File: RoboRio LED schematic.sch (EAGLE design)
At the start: 5 parts

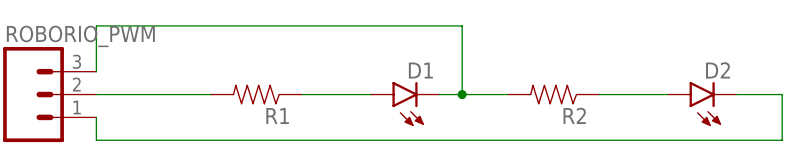
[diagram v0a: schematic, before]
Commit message: Jordan - RoboRio LED fixed
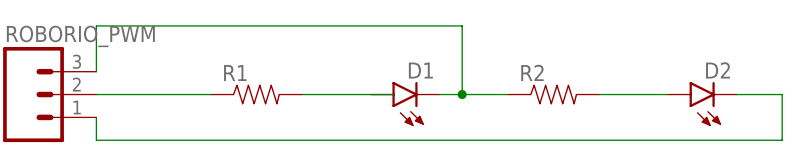
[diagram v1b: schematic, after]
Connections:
- removed net 6V: R1.2, ROBORIO_PWM.2
- removed net N$3: D2.A, R2.1
- new net N$2: R1.2
- new net N$4: D2.A, R2.2
- net N$1: now also ROBORIO_PWM.2; no longer D1.A
- net S: now also R2.1; no longer R2.2
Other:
- moved on the sheet: R1, R2
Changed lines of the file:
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@@
 <instance part="D1" gate="G$1" x="-12.7" y="60.96" rot="R90"/>
 <instance part="D2" gate="G$1" x="20.32" y="60.96" rot="R90"/>
-<instance part="R1" gate="G$1" x="-27.94" y="60.96" rot="R180"/>
-<instance part="R2" gate="G$1" x="5.08" y="60.96" rot="R180"/>
+<instance part="R1" gate="G$1" x="-27.94" y="60.96"/>
+<instance part="R2" gate="G$1" x="5.08" y="60.96"/>
 </instances>
 <busses>
 </busses>
 <nets>
-<net name="N$1" class="0">
-<segment>
-<pinref part="R1" gate="G$1" pin="1"/>
-<pinref part="D1" gate="G$1" pin="A"/>
-<wire x1="-22.86" y1="60.96" x2="-15.24" y2="60.96" width="0.1524" layer="91"/>
-</segment>
-</net>
 <net name="S" class="0">
 <segment>
-<pinref part="D1" gate="G$1" pin="C"/>
-<pinref part="R2" gate="G$1" pin="2"/>
-<wire x1="-7.62" y1="60.96" x2="-5.08" y2="60.96" width="0.1524" layer="91"/>
 <pinref part="ROBORIO_PWM" gate="J$1" pin="3"/>
-<wire x1="-5.08" y1="60.96" x2="0" y2="60.96" width="0.1524" layer="91"/>
 <wire x1="-45.72" y1="63.5" x2="-45.72" y2="68.58" width="0.1524" layer="91"/>
 <wire x1="-45.72" y1="68.58" x2="-5.08" y2="68.58" width="0.1524" layer="91"/>
+<pinref part="D1" gate="G$1" pin="C"/>
+<pinref part="R2" gate="G$1" pin="1"/>
+<wire x1="-7.62" y1="60.96" x2="-5.08" y2="60.96" width="0.1524" layer="91"/>
+<wire x1="-5.08" y1="60.96" x2="0" y2="60.96" width="0.1524" layer="91"/>
 <wire x1="-5.08" y1="68.58" x2="-5.08" y2="60.96" width="0.1524" layer="91"/>
 <junction x="-5.08" y="60.96"/>
-</segment>
-</net>
-<net name="N$3" class="0">
-<segment>
-<pinref part="R2" gate="G$1" pin="1"/>
-<pinref part="D2" gate="G$1" pin="A"/>
-<wire x1="10.16" y1="60.96" x2="17.78" y2="60.96" width="0.1524" layer="91"/>
-</segment>
-</net>
-<net name="6V" class="0">
-<segment>
-<pinref part="ROBORIO_PWM" gate="J$1" pin="2"/>
-<pinref part="R1" gate="G$1" pin="2"/>
-<wire x1="-45.72" y1="60.96" x2="-33.02" y2="60.96" width="0.1524" layer="91"/>
 </segment>
 </net>
@@
 </segment>
 </net>
+<net name="N$1" class="0">
+<segment>
+<pinref part="ROBORIO_PWM" gate="J$1" pin="2"/>
+<pinref part="R1" gate="G$1" pin="1"/>
+<wire x1="-45.72" y1="60.96" x2="-33.02" y2="60.96" width="0.1524" layer="91"/>
+</segment>
+</net>
+<net name="N$2" class="0">
+<segment>
+<pinref part="R1" gate="G$1" pin="2"/>
+<wire x1="-22.86" y1="60.96" x2="-12.7" y2="60.96" width="0.1524" layer="91"/>
+</segment>
+</net>
+<net name="N$4" class="0">
+<segment>
+<pinref part="R2" gate="G$1" pin="2"/>
+<pinref part="D2" gate="G$1" pin="A"/>
+<wire x1="10.16" y1="60.96" x2="17.78" y2="60.96" width="0.1524" layer="91"/>
+</segment>
+</net>

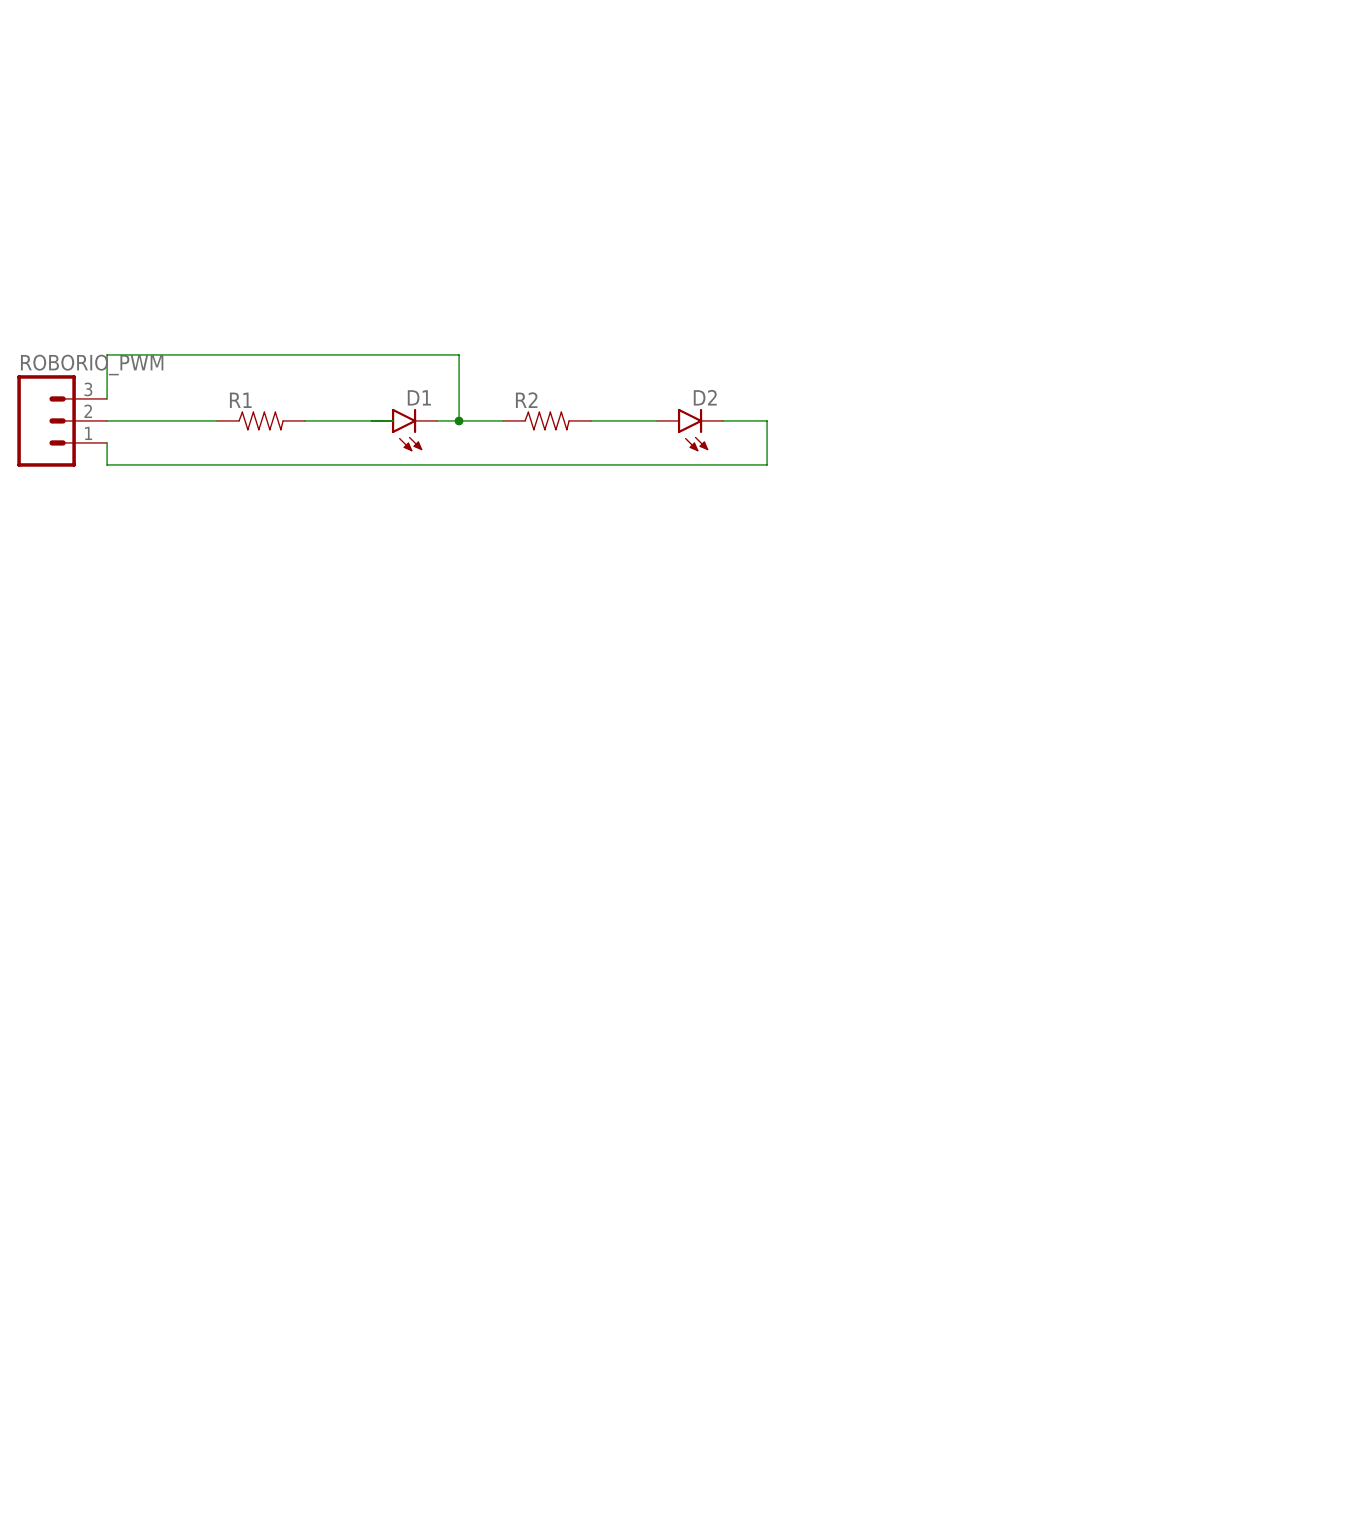
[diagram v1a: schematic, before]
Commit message: Jordan RoboRio LED Final
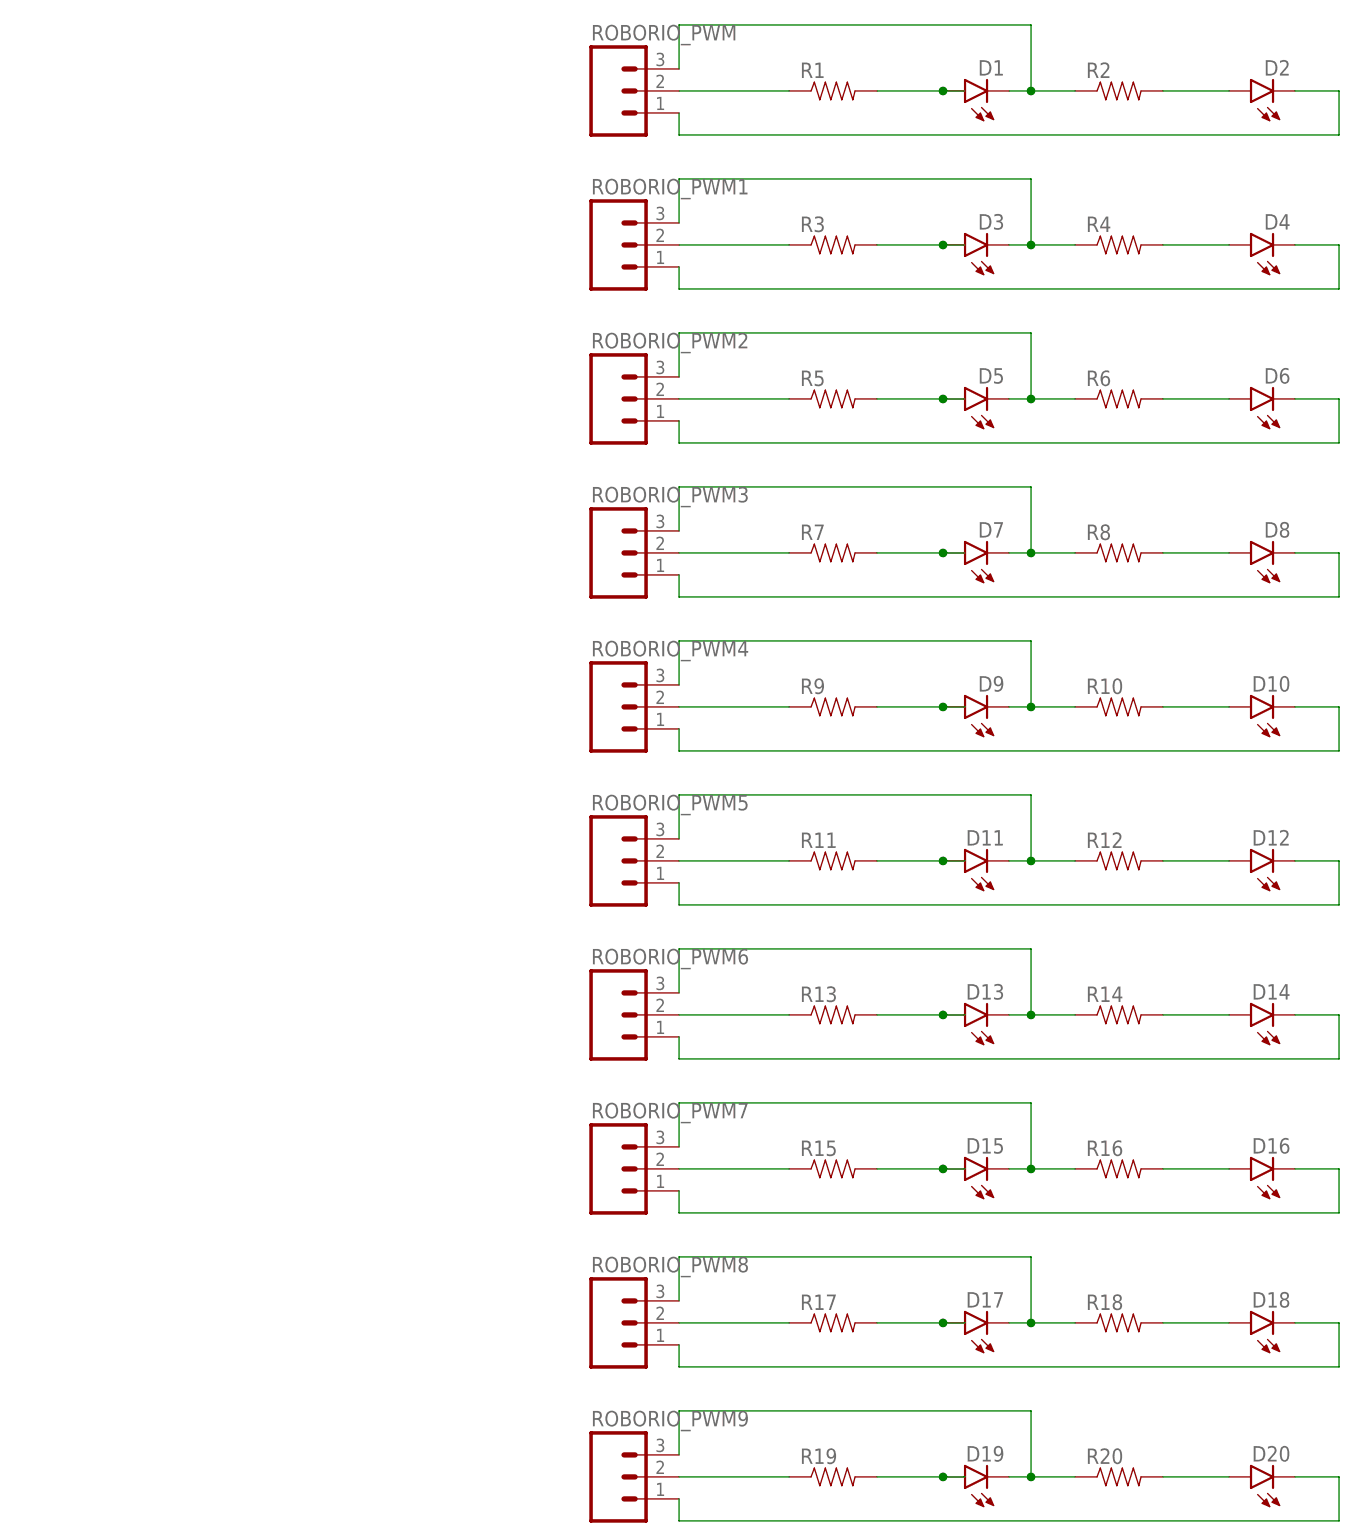
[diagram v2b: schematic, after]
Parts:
- added D10, D11, D12, D13, D14, D15, D16, D17, D18, D19, D20, D3, D4, D5, D6, D7, D8, D9: (no value), SparkFun-LED:LED5MM
- added R10, R11, R12, R13, R14, R15, R16, R17, R18, R19, R20, R3, R4, R5, R6, R7, R8, R9: (no value), SparkFun-Passives:RESISTOR1206
- added ROBORIO_PWM1, ROBORIO_PWM2, ROBORIO_PWM3, ROBORIO_PWM4, ROBORIO_PWM5, ROBORIO_PWM6, ROBORIO_PWM7, ROBORIO_PWM8, ROBORIO_PWM9: (no value), SparkFun-Connectors:M03POGO_PIN_HOLES_ONLY
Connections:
- new net GND1: D4.C, ROBORIO_PWM1.1
- new net GND2: D6.C, ROBORIO_PWM2.1
- new net GND3: D8.C, ROBORIO_PWM3.1
- new net GND4: D10.C, ROBORIO_PWM4.1
- new net GND5: D12.C, ROBORIO_PWM5.1
- new net GND6: D14.C, ROBORIO_PWM6.1
- new net GND7: D16.C, ROBORIO_PWM7.1
- new net GND8: D18.C, ROBORIO_PWM8.1
- new net GND9: D20.C, ROBORIO_PWM9.1
- new net N$10: R7.1, ROBORIO_PWM3.2
- new net N$11: D7.A, R7.2
- new net N$12: D8.A, R8.2
- new net N$13: R9.1, ROBORIO_PWM4.2
- new net N$14: D9.A, R9.2
- new net N$15: D10.A, R10.2
- new net N$16: R11.1, ROBORIO_PWM5.2
- new net N$17: D11.A, R11.2
- new net N$18: D12.A, R12.2
- new net N$19: R13.1, ROBORIO_PWM6.2
- new net N$20: D13.A, R13.2
- new net N$21: D14.A, R14.2
- new net N$22: R15.1, ROBORIO_PWM7.2
- new net N$23: D15.A, R15.2
- new net N$24: D16.A, R16.2
- new net N$25: R17.1, ROBORIO_PWM8.2
- new net N$26: D17.A, R17.2
- new net N$27: D18.A, R18.2
- new net N$28: R19.1, ROBORIO_PWM9.2
- new net N$29: D19.A, R19.2
- new net N$3: R3.1, ROBORIO_PWM1.2
- new net N$30: D20.A, R20.2
- new net N$5: D3.A, R3.2
- new net N$6: D4.A, R4.2
- new net N$7: R5.1, ROBORIO_PWM2.2
- new net N$8: D5.A, R5.2
- new net N$9: D6.A, R6.2
- new net S1: D3.C, R4.1, ROBORIO_PWM1.3
- new net S2: D5.C, R6.1, ROBORIO_PWM2.3
- new net S3: D7.C, R8.1, ROBORIO_PWM3.3
- new net S4: D9.C, R10.1, ROBORIO_PWM4.3
- new net S5: D11.C, R12.1, ROBORIO_PWM5.3
- new net S6: D13.C, R14.1, ROBORIO_PWM6.3
- new net S7: D15.C, R16.1, ROBORIO_PWM7.3
- new net S8: D17.C, R18.1, ROBORIO_PWM8.3
- new net S9: D19.C, R20.1, ROBORIO_PWM9.3
- net N$2: now also D1.A
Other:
- moved on the sheet: D1, D2, R1, R2, ROBORIO_PWM
